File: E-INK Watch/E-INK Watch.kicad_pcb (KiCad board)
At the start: 2 copper layers, 31.8 x 36.8 mm, 53 parts, among them J1 Conn_01x04_Female, J2 USB_B_Micro, J3 JST PH, J4 EINK, Q1 DMG2305UX-13, Q2 AO3418, T1 BSS806NEH6327XTSA1, U1 PIC18F27J53_ISS, U2 DPS310, U3 MCP73831-2-OT, U4 S-1318B33-M5T1U4, Y1 32.768kHz

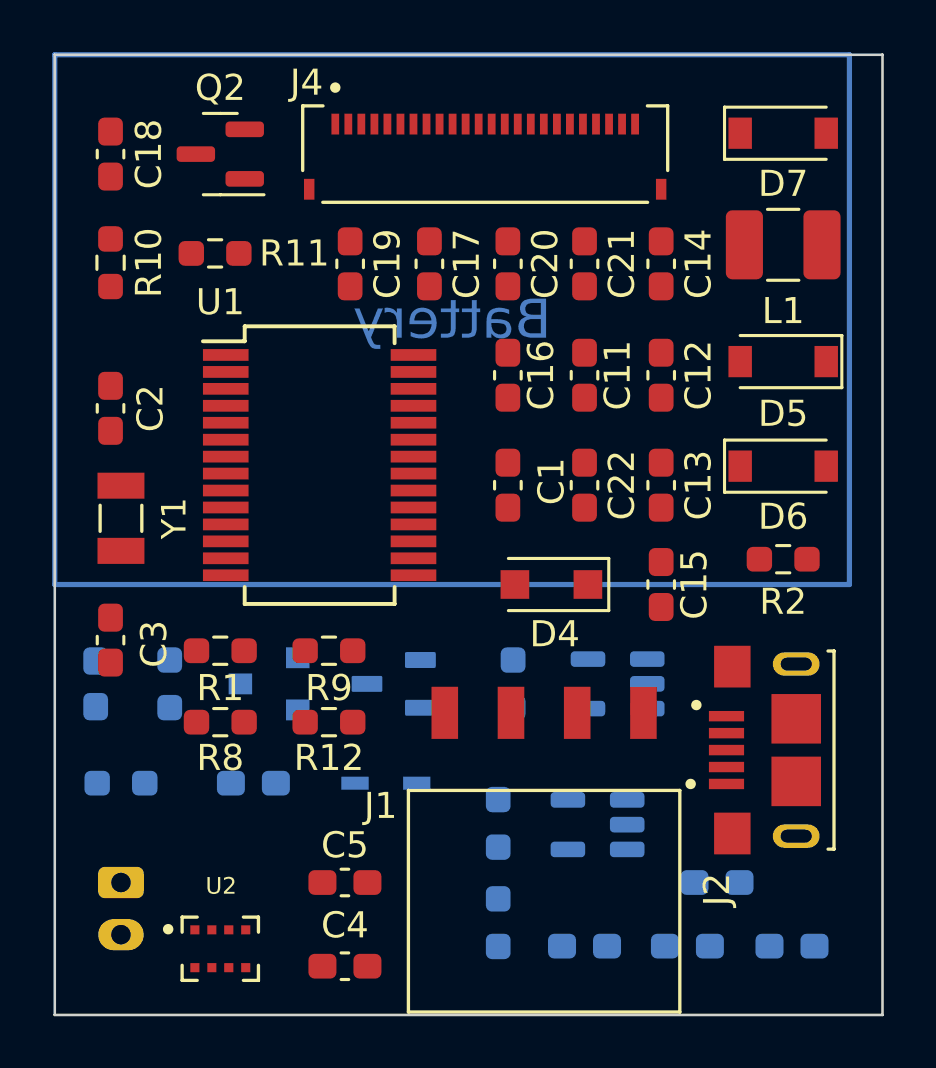
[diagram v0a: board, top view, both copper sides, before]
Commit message: Completed PCB and gerber files
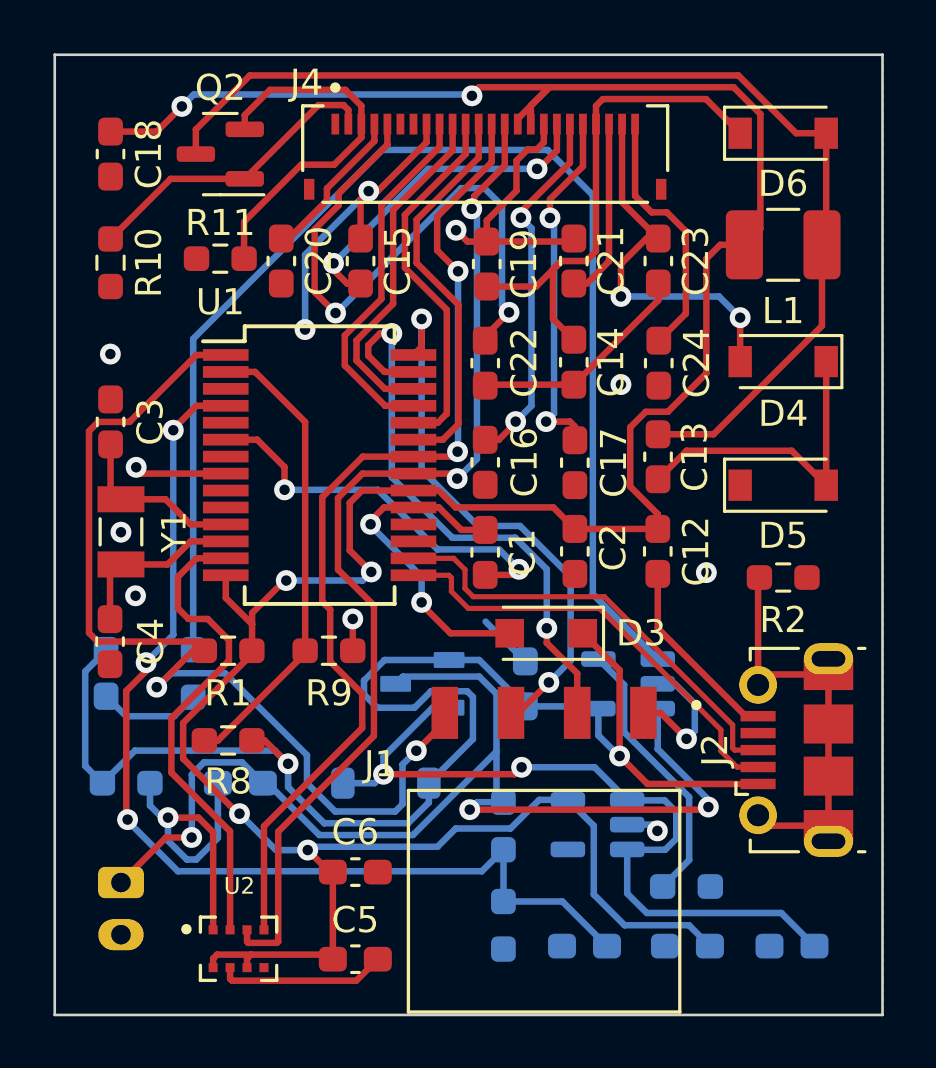
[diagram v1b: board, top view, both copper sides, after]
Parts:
- removed the C13 at (103.3, 116.8)
- removed the C3 at (82.2, 122.8)
- removed R12: 510k 0.1%, Resistor_SMD:R_0603_1608Metric_Pad0.98x0.95mm_HandSolder
- removed T1: BSS806NEH6327XTSA1, e-ink:DIO_BB914E6327HTSA1
- added C22: 4.7uF, Capacitor_SMD:C_0603_1608Metric_Pad1.08x0.95mm_HandSolder, F.Cu at (96.5, 112.2)
- added C23: 4.7uF, Capacitor_SMD:C_0603_1608Metric_Pad1.08x0.95mm_HandSolder, F.Cu at (103.2, 108.2)
- added C24: 1uF, Capacitor_SMD:C_0603_1608Metric_Pad1.08x0.95mm_HandSolder, F.Cu at (103.2, 112.2)
- added C6: 100nF, Capacitor_SMD:C_0603_1608Metric_Pad1.08x0.95mm_HandSolder, F.Cu at (91.5, 131.7)
- C13: renamed from C12; value 1uF -> 4.7uF
- C17, C19, C21: value 1uF -> 4.7uF
- C4: value 100nF -> 7pF
- D2: renamed from D3; value SD103AWS-TP -> SD103AW-13-F; footprint e-ink:SOD2512X115N -> Diode_SMD:D_SOD-123
- J2: footprint e-ink:AMPHENOL_10118193-0001LF -> Connector_USB:USB_Micro-B_Molex-105017-0001
- L1: value 47uH -> 10uH
- R11: value 2R2 -> 0.47R
- R3: renamed from R5; value 150 -> 150R
- R9: value 0R -> 510k 0.1%
- moved C15 16.9 mm to (91.7, 108.2)
- moved C4 15.4 mm to (82.1, 122.8), turned to 90 degrees
- moved C7 10.6 mm to (98.1, 124.5), turned to 90 degrees
- moved R4 10.2 mm to (104.2, 132.2), turned to 180 degrees
- moved C17 9.45 mm to (100.0, 116.0), turned to 90 degrees
- moved C20 8.69 mm to (88.7, 108.2), turned to 90 degrees
- moved C12 7.32 mm to (103.1, 119.4)
- moved C19 5.24 mm to (96.6, 108.4)
- moved C14 5.05 mm to (99.9, 112.1)
- moved C1 4.60 mm to (96.5, 119.4)
- moved C2 3.61 mm to (100.0, 119.4)
- moved C16 3.45 mm to (96.5, 116.0), turned to 90 degrees
- moved C13 3.13 mm to (103.2, 115.8)
- moved C5 2.97 mm to (91.5, 135.0)
- moved D3 1.88 mm to (98.9, 122.5)
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- renumbered C22 to C1, C9 to C10, C10 to C11, C11 to C12, C1 to C2, C2 to C3, C6 to C7, C7 to C8, C8 to C9, D2 to D1, D4 to D3, D5 to D4, D6 to D5, D7 to D6, R3 to R4, R6 to R5, R4 to R6
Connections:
- net /D/C# renamed /D/C
- net /RES# renamed /RES
- C12 pad 2: /Screen/VDD -> +3.3V
- C15 pad 1: +3.3V -> GND
- C15 pad 2: GND -> Net-(J4-VDD)
- C16 pad 1: /Screen/VDD -> GND
- C16 pad 2: GND -> Net-(J4-VPP)
- C17 pad 1: Net-(C17-Pad1) -> GND
- C17 pad 2: GND -> Net-(J4-VSH)
- C18 pad 2: Net-(C18-Pad2) -> +3.3V
- C19 pad 1: Net-(C19-Pad1) -> GND
- C19 pad 2: GND -> /Screen/PREVGH
- C20 pad 1: Net-(C20-Pad1) -> GND
- C20 pad 2: GND -> Net-(J4-VGL)
- C21 pad 1: Net-(C21-Pad1) -> GND
- C21 pad 2: GND -> Net-(J4-VSL)
- C4 pad 2: +3.3V -> /OSC2
- C9 pad 1: Net-(C8-Pad1) -> Net-(D2-K)
- D5 pad 1: Net-(C13-Pad2) -> GND
- J4 pad 18: /Screen/VDD -> Net-(J4-VDD)
- J4 pad 19: GND -> Net-(J4-VPP)
- J4 pad 20: Net-(C17-Pad1) -> Net-(J4-VSH)
- J4 pad 22: Net-(C20-Pad1) -> Net-(J4-VSL)
- J4 pad 24: Net-(C21-Pad1) -> Net-(J4-VCOM)
- J4 pad 4: Net-(C18-Pad2) -> Net-(J4-VGL)
- J4 pad 5: Net-(C19-Pad1) -> Net-(J4-VGH)
- L1 pad 1: /Screen/VDD -> +3.3V
- Q1 pad 2: Net-(Q1-Pad2) -> Net-(D2-K)
- R2 pad 2: Net-(J2-Pad6) -> Net-(J2-Shield)
- R9 pad 1: /Screen/VDD -> GND
- R9 pad 2: +3.3V -> /USB_IN
- U1 pad 3: /BATT_OFF -> unconnected-(U1-RA1/AN1-Pad3)
- U4 pad 1: Net-(C8-Pad1) -> Net-(D2-K)
- U4 pad 3: Net-(C8-Pad1) -> Net-(D2-K)
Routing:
- net +3.3V: track 0.00 -> 116.0 mm, vias 0 -> 6
- net GND: track 0.00 -> 84.5 mm, vias 0 -> 15
- net +5V: track 0.00 -> 55.9 mm, vias 0 -> 2
- net Net-(U3-STAT): track 0.00 -> 49.8 mm
- net +BATT: track 0.00 -> 43.9 mm, vias 0 -> 3
- net Net-(D6-A): track 0.00 -> 42.4 mm
- net /SDI: track 0.00 -> 40.7 mm, vias 0 -> 2
- net /BATT_V: track 0.00 -> 40.6 mm, vias 0 -> 3
- net /SCK: track 0.00 -> 38.7 mm, vias 0 -> 2
- net /~{MCLR}: track 0.00 -> 38.2 mm, vias 0 -> 2
- net Net-(D2-K): track 0.00 -> 30.5 mm, vias 0 -> 2
- net Net-(J4-VGH): track 0.00 -> 23.1 mm, vias 0 -> 2
- net /ISCPCLK: track 0.00 -> 22.6 mm, vias 0 -> 2
- net /ISCPDAT: track 0.00 -> 21.1 mm, vias 0 -> 2
- net /Screen/PREVGH: track 0.00 -> 20.0 mm
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- added copper zone on F.Cu, net GND
- removed copper zone on F.Cu, net +3.3V
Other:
- board text added: "C13"
- board text removed: "Battery"
